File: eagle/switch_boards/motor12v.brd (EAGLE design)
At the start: 93 x 16.5 mm, 9 parts

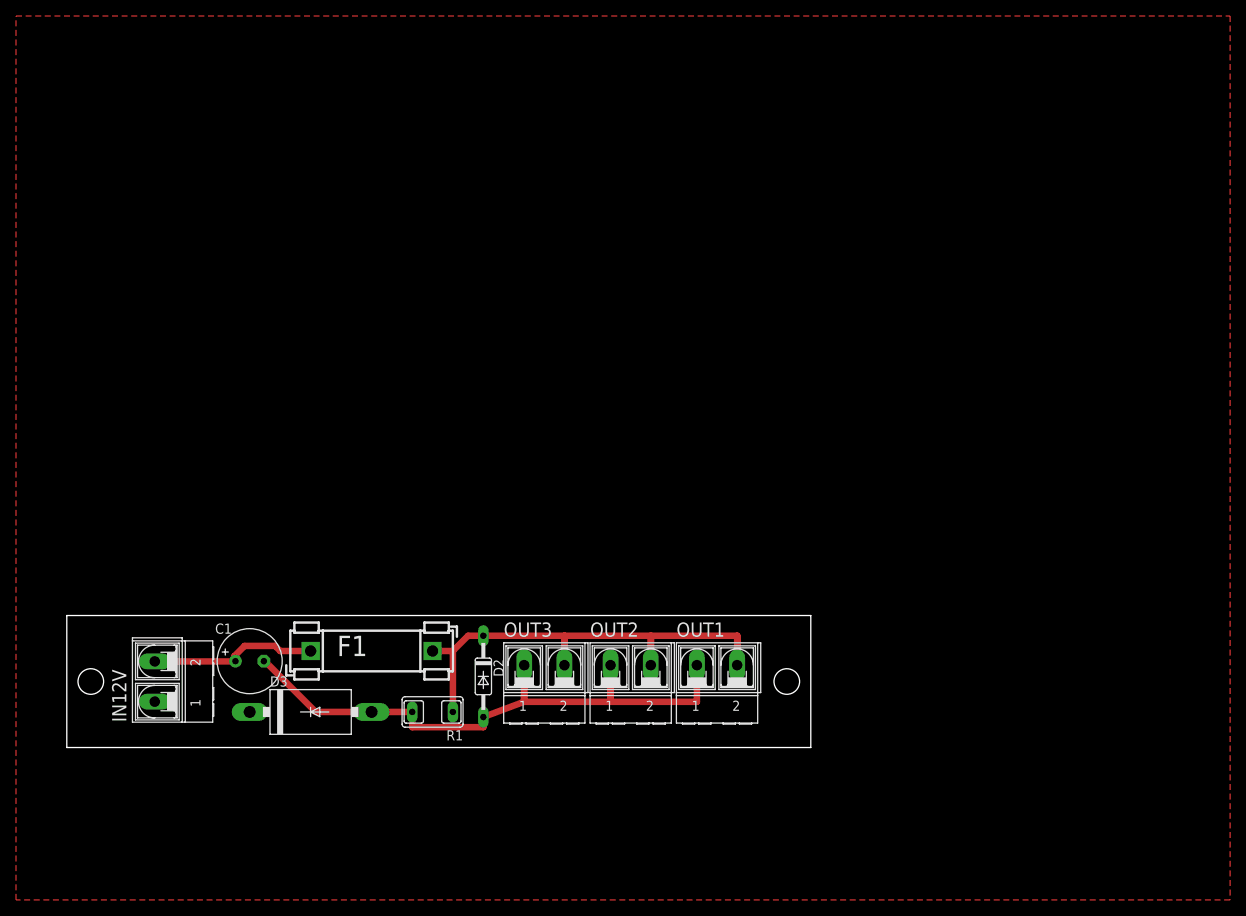
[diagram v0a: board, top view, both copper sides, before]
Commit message: Motor switch board ver.  2.0
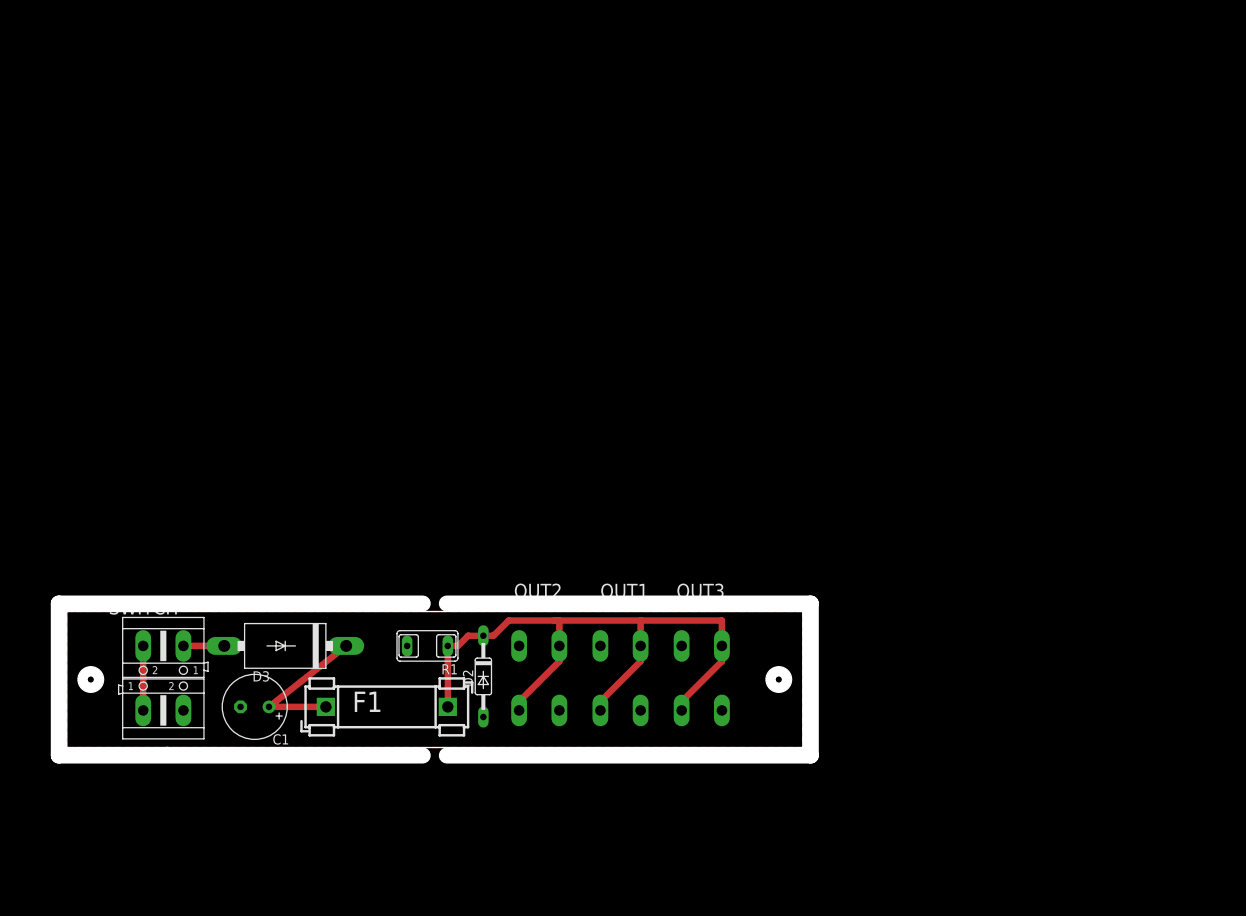
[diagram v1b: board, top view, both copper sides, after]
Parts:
- added OUT4, OUT5, OUT6, SWITCH: (no value), con-ptr500:AK500/2
- C1: value (none) -> 100uF
- IN12V, OUT1, OUT2, OUT3: device con-ptr500:AK500/2-H -> con-ptr500:AK500/2
- moved OUT3 19.8 mm to (79.4, 12.7), flipped to the bottom, turned to 180 degrees
- moved OUT1 12.3 mm to (69.2, 12.7), flipped to the bottom, turned to 180 degrees
- moved OUT2 11.7 mm to (59.1, 12.7), flipped to the bottom, turned to 180 degrees
- moved D3 8.84 mm to (27.3, 12.7), turned to 180 degrees
- moved R1 8.28 mm to (45.1, 12.7)
- moved F1 7.24 mm to (32.4, 5.08)
- moved C1 5.75 mm to (23.5, 5.08), turned to 180 degrees
- moved IN12V 3.77 mm to (12.1, 4.63), turned to 0 degrees
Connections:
- removed net OUT_GND: C1.-, D2.A, D3.A, OUT1.1, OUT2.1, OUT3.1, R1.2
- new net EN21: C1.+, D3.C, F1.1
- new net IN12V: D3.A, SWITCH.1
- net +12V: now also IN12V.1, SWITCH.2; no longer C1.+, F1.1, IN12V.2
- net GND: now also C1.-, D2.A, IN12V.2, OUT1.1, OUT2.1, OUT3.1, OUT4.1, OUT5.1, OUT6.1, R1.2; no longer D3.C, IN12V.1
- net OUT_+12V: now also OUT4.2, OUT5.2, OUT6.2
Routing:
- net OUT_GND: track 87.7 -> 0.00 mm
- net EN21: track 0.00 -> 19.4 mm
- net OUT_+12V: track 68.5 -> 83.8 mm
- net +12V: track 21.1 -> 8.07 mm
- net IN12V: track 0.00 -> 5.11 mm
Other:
- board size 93 x 16.5 mm -> 94 x 19 mm
